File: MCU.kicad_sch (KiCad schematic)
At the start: 45 parts, among them IC3 TCAN330DCNT, J1 BM04B-GHS-TBT_LF__SN__N_, J2 Conn_01x04_Pin, J3 USB_C_Receptacle_USB2.0_16P, J4 BM04B-GHS-TBT_LF__SN__N_, J5 Conn_01x02_Socket, SW1 SW_SPDT, SW2 SW_SPDT, U2 STM32G431CBU6, U3 ME6211C33M5, Y1 ECS-80-20-5PX-TR

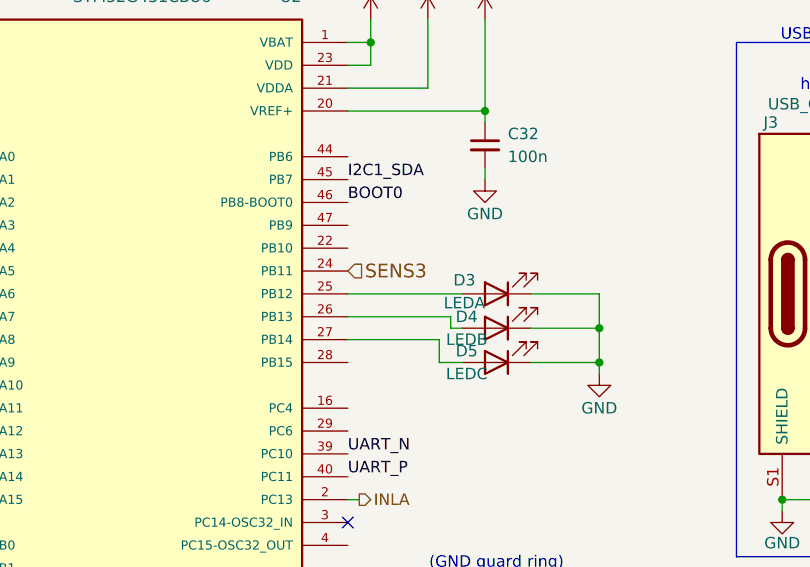
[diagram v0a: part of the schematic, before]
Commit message: new pcb
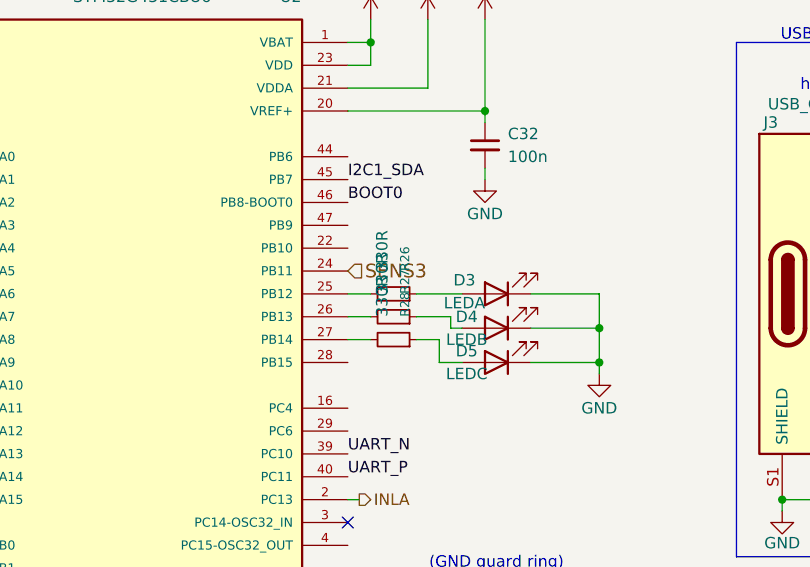
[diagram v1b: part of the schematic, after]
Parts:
- added R26, R27, R28: 330R, Resistor_SMD:R_0603_1608Metric_Pad0.98x0.95mm_HandSolder, symbol Device:R_Small
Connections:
- net at D5.2 (A): now also R28.1; no longer U2.27 (PB14)
- net at D4.2 (A): now also R27.1; no longer U2.26 (PB13)
- net at D3.2 (A): now also R26.1; no longer U2.25 (PB12)
- new net: R27.2, U2.26 (PB13)
- new net: R26.2, U2.25 (PB12)
- new net: R28.2, U2.27 (PB14)
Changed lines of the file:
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@@
 	(wire
 		(pts
+			(xy 157.48 85.09) (xy 154.94 85.09)
+		)
+		(stroke
+			(width 0)
+			(type default)
+		)
+	)
+	(wire
+		(pts
 			(xy 175.26 86.36) (xy 182.88 86.36)
 		)
@@
 	(wire
 		(pts
+			(xy 157.48 87.63) (xy 154.94 87.63)
+		)
+		(stroke
+			(width 0)
+			(type default)
+		)
+	)
+	(wire
+		(pts
 			(xy 165.1 90.17) (xy 165.1 87.63)
 		)
@@
 	(wire
 		(pts
-			(xy 154.94 82.55) (xy 167.64 82.55)
+			(xy 154.94 82.55) (xy 157.48 82.55)
 		)
 		(stroke
@@
 	(wire
 		(pts
+			(xy 162.56 82.55) (xy 167.64 82.55)
+		)
+		(stroke
+			(width 0)
+			(type default)
+		)
+	)
+	(wire
+		(pts
 			(xy 234.95 119.38) (xy 232.41 119.38)
 		)
@@
 	(wire
 		(pts
-			(xy 165.1 87.63) (xy 154.94 87.63)
+			(xy 165.1 87.63) (xy 162.56 87.63)
 		)
 		(stroke
@@
 	(wire
 		(pts
-			(xy 166.37 85.09) (xy 154.94 85.09)
+			(xy 166.37 85.09) (xy 162.56 85.09)
 		)
 		(stroke
@@
 	)
 	(symbol
+		(lib_id "Device:R_Small")
+		(at 160.02 85.09 270)
+		(mirror x)
+		(unit 1)
+		(exclude_from_sim no)
+		(in_bom yes)
+		(on_board yes)
+		(dnp no)
+		(fields_autoplaced yes)
+		(property "Reference" "R27"
+			(at 161.2901 82.55 0)
+			(effects
+				(font
+					(size 1.016 1.016)
+				)
+				(justify left)
+			)
+		)
+		(property "Value" "330R"
+			(at 158.7501 82.55 0)
+			(effects
+				(font
+					(size 1.27 1.27)
+				)
+				(justify left)
+			)
+		)
+		(property "Footprint" "Resistor_SMD:R_0603_1608Metric_Pad0.98x0.95mm_HandSolder"
+			(at 160.02 85.09 0)
+			(effects
+				(font
+					(size 1.27 1.27)
+				)
+				(hide yes)
+			)
+		)
+		(property "Datasheet" "~"
+			(at 160.02 85.09 0)
+			(effects
+				(font
+					(size 1.27 1.27)
+				)
+				(hide yes)
+			)
+		)
+		(property "Description" "Resistor, small symbol"
+			(at 160.02 85.09 0)
+			(effects
+				(font
+					(size 1.27 1.27)
+				)
+				(hide yes)
+			)
+		)
+		(pin "1"
+		)
+		(pin "2"
+		)
+		(instances
+			(project "Ana_ESC"
+				(path "/57129761-6d47-486c-bd7a-90dbb6f75754/223db1af-68f5-46b9-9722-256b09606f21"
+					(reference "R27")
+					(unit 1)
+				)
+			)
+		)
+	)
+	(symbol
 		(lib_id "power:GND")
 		(at 196.85 40.64 0)
@@
 	)
 	(symbol
+		(lib_id "Device:R_Small")
+		(at 160.02 82.55 270)
+		(mirror x)
+		(unit 1)
+		(exclude_from_sim no)
+		(in_bom yes)
+		(on_board yes)
+		(dnp no)
+		(fields_autoplaced yes)
+		(property "Reference" "R26"
+			(at 161.2901 80.01 0)
+			(effects
+				(font
+					(size 1.016 1.016)
+				)
+				(justify left)
+			)
+		)
+		(property "Value" "330R"
+			(at 158.7501 80.01 0)
+			(effects
+				(font
+					(size 1.27 1.27)
+				)
+				(justify left)
+			)
+		)
+		(property "Footprint" "Resistor_SMD:R_0603_1608Metric_Pad0.98x0.95mm_HandSolder"
+			(at 160.02 82.55 0)
+			(effects
+				(font
+					(size 1.27 1.27)
+				)
+				(hide yes)
+			)
+		)
+		(property "Datasheet" "~"
+			(at 160.02 82.55 0)
+			(effects
+				(font
+					(size 1.27 1.27)
+				)
+				(hide yes)
+			)
+		)
+		(property "Description" "Resistor, small symbol"
+			(at 160.02 82.55 0)
+			(effects
+				(font
+					(size 1.27 1.27)
+				)
+				(hide yes)
+			)
+		)
+		(pin "1"
+		)
+		(pin "2"
+		)
+		(instances
+			(project "Ana_ESC"
+				(path "/57129761-6d47-486c-bd7a-90dbb6f75754/223db1af-68f5-46b9-9722-256b09606f21"
+					(reference "R26")
+					(unit 1)
+				)
+			)
+		)
+	)
+	(symbol
 		(lib_id "power:GND")
 		(at 82.55 38.1 0)
@@
 					(unit 1)
 				)
+			)
+		)
+	)
+	(symbol
+		(lib_id "Device:R_Small")
+		(at 160.02 87.63 270)
+		(mirror x)
+		(unit 1)
+		(exclude_from_sim no)
+		(in_bom yes)
+		(on_board yes)
+		(dnp no)
+		(fields_autoplaced yes)
+		(property "Reference" "R28"
+			(at 161.2901 85.09 0)
+			(effects
+				(font
+					(size 1.016 1.016)
+				)
+				(justify left)
+			)
+		)
+		(property "Value" "330R"
+			(at 158.7501 85.09 0)
+			(effects
+				(font
+					(size 1.27 1.27)
+				)
+				(justify left)
+			)
+		)
+		(property "Footprint" "Resistor_SMD:R_0603_1608Metric_Pad0.98x0.95mm_HandSolder"
+			(at 160.02 87.63 0)
+			(effects
+				(font
+					(size 1.27 1.27)
+				)
+				(hide yes)
+			)
+		)
+		(property "Datasheet" "~"
+			(at 160.02 87.63 0)
+			(effects
+				(font
+					(size 1.27 1.27)
+				)
+				(hide yes)
+			)
+		)
+		(property "Description" "Resistor, small symbol"
+			(at 160.02 87.63 0)
+			(effects
+				(font
+					(size 1.27 1.27)
+				)
+				(hide yes)
+			)
+		)
+		(pin "1"
+		)
+		(pin "2"
+		)
+		(instances
+			(project "Ana_ESC"
+				(path "/57129761-6d47-486c-bd7a-90dbb6f75754/223db1af-68f5-46b9-9722-256b09606f21"
+					(reference "R28")
+					(unit 1)
+				)
